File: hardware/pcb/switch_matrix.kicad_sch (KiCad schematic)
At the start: 38 parts, among them SW1 SW_Push, SW10 SW_Push, SW11 SW_Push, SW12 SW_Push, SW13 SW_Push, SW14 SW_Push, SW15 SW_Push, SW16 SW_Push, SW2 SW_Push, SW3 SW_Push, SW4 SW_Push, SW5 SW_Push, SW6 SW_Push, SW7 SW_Push, SW8 SW_Push, SW9 SW_Push

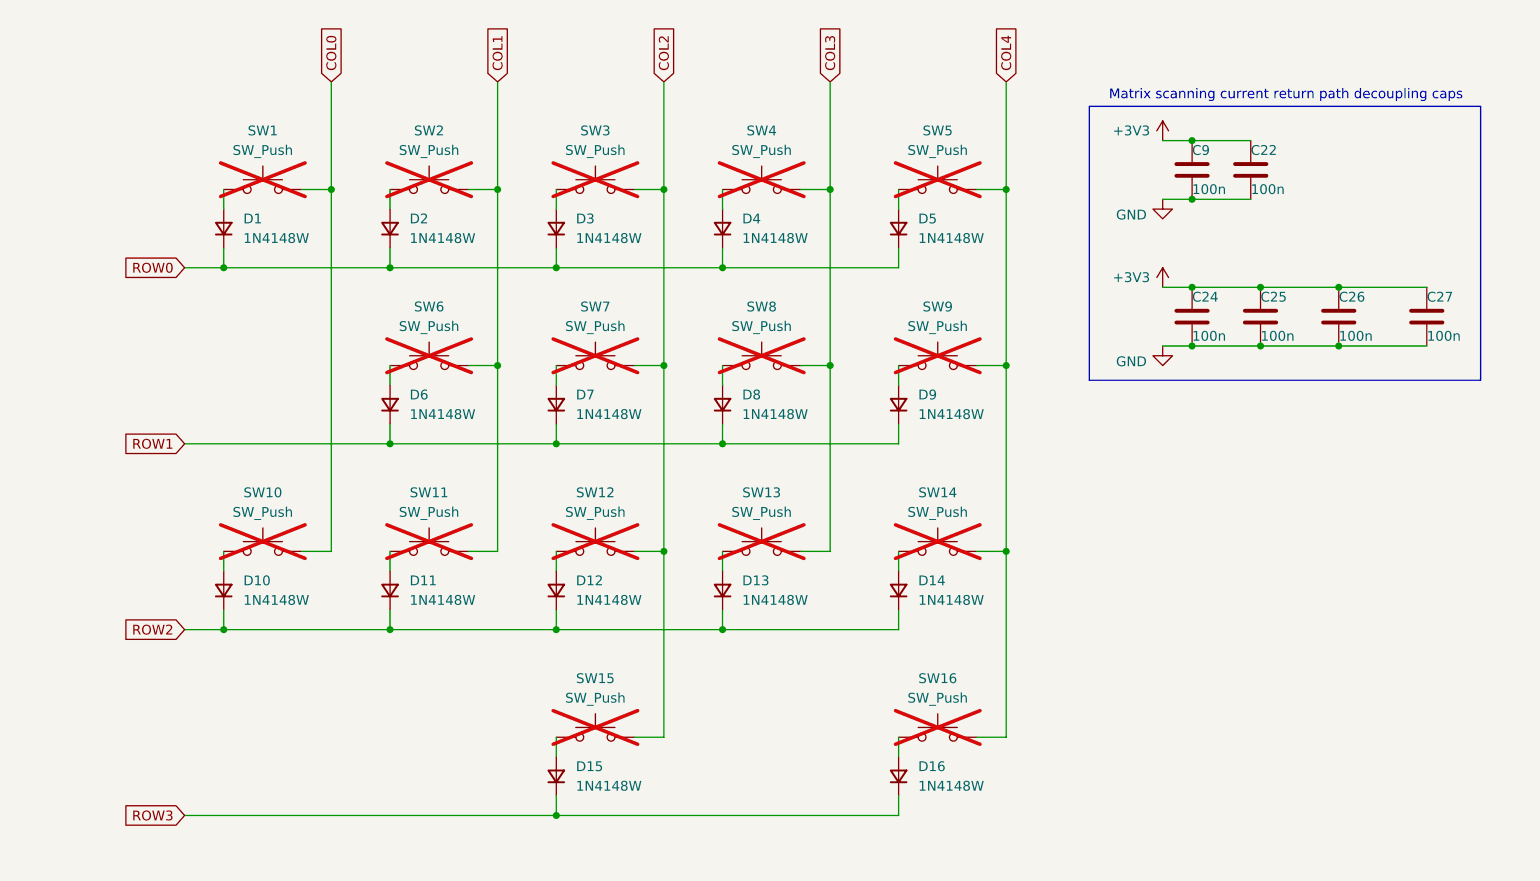
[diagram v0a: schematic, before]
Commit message: Version 1.5
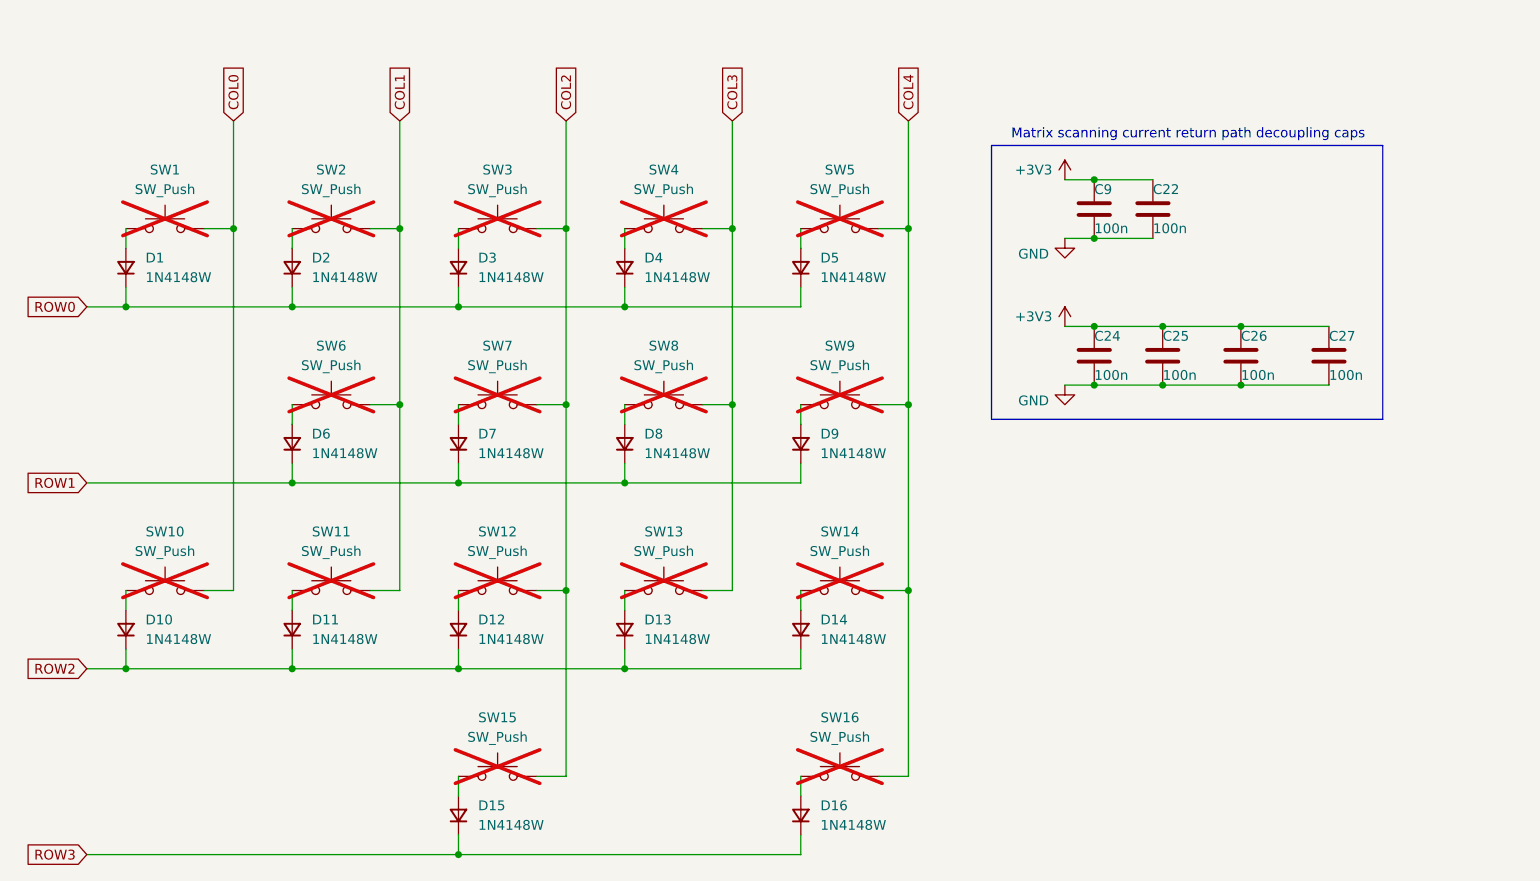
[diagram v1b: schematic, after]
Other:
- moved on the sheet: C22, C24, C25, C26, C27, C9, D1, D10, D11, D12, D13, D14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
